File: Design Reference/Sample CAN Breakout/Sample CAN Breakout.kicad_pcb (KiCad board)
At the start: 2 copper layers, 7 parts, among them J1 2604-1102, J2 2604-1102, J3 2604-1102, J4 2604-1102, J5 2604-1102, J6 2604-1102, J7 2604-1102

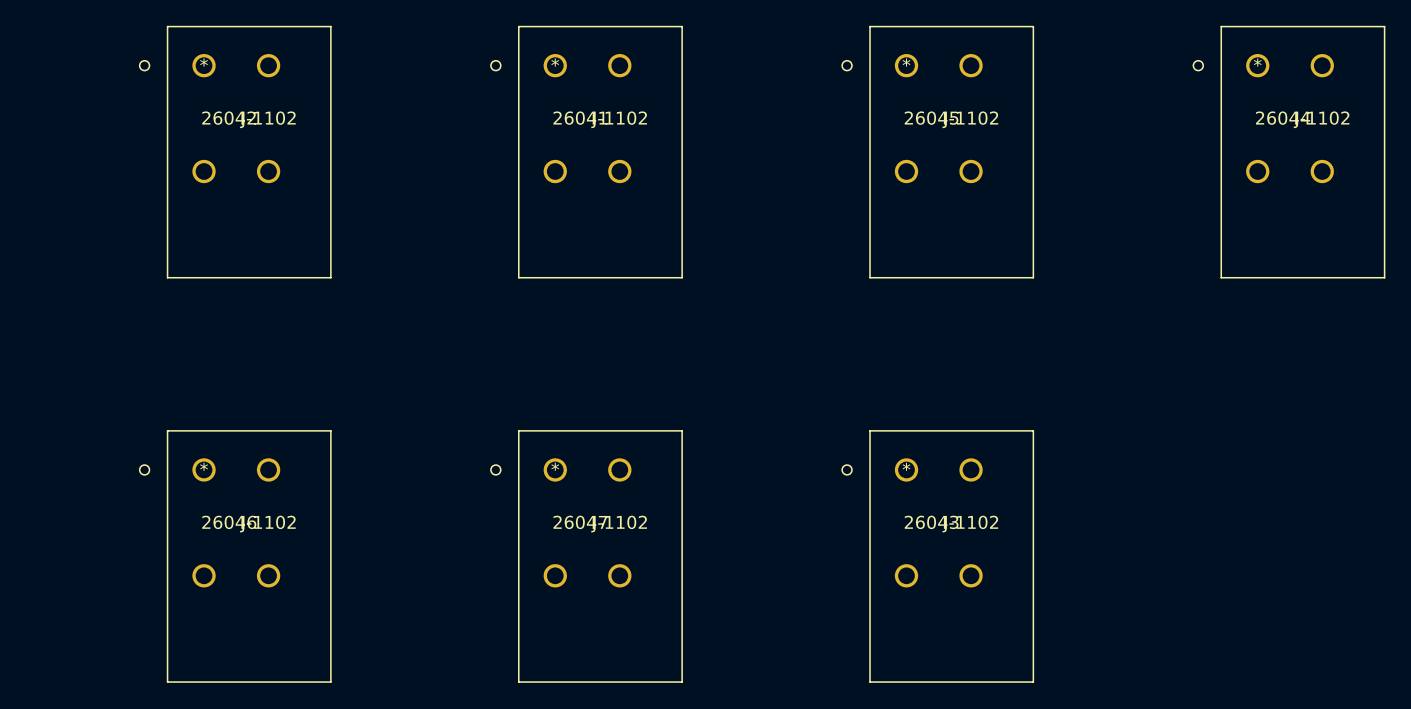
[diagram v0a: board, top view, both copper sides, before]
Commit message: Reference Design 1 Finished
Ruler Reference Design Finished
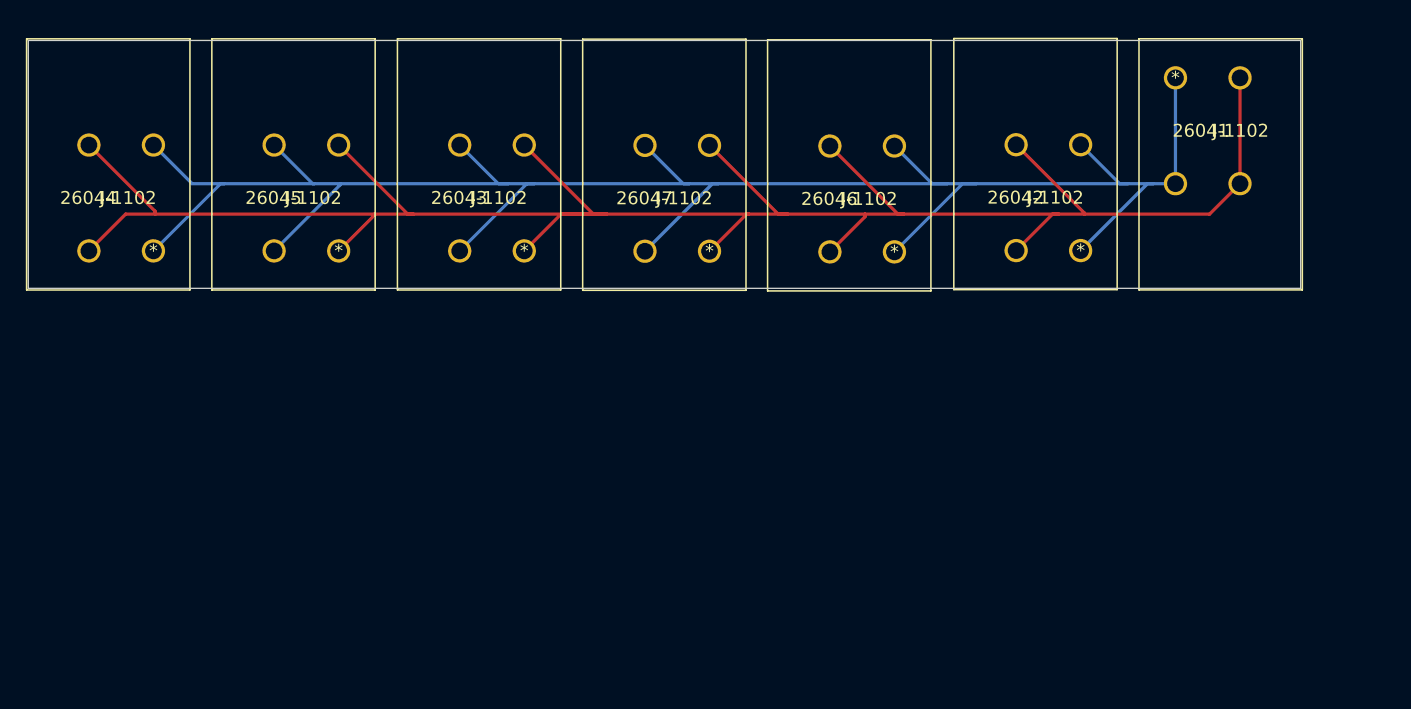
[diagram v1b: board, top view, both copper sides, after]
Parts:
- moved J4 86.7 mm to (97.9, 96.9), turned to 180 degrees
- moved J2 69.4 mm to (169.7, 96.8), turned to 180 degrees
- moved J6 56.1 mm to (155.3, 96.9), turned to 180 degrees
- moved J1 48.1 mm to (177.0, 83.4)
- moved J5 46.3 mm to (112.2, 96.9), turned to 180 degrees
- moved J3 34.1 mm to (126.6, 96.9), turned to 180 degrees
- moved J7 20.7 mm to (140.9, 96.9), turned to 180 degrees
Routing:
- net Net-(J1-Pad3): track 0.00 -> 171.7 mm
- net Net-(J1-Pad1): track 0.00 -> 159.9 mm
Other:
- board outline added: 98.6 x 19.2 mm
